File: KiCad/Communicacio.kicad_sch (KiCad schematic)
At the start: 11 parts, among them J2 USB_B_Micro, J3 Conn_PIC_ICSP_ICD, SW2 SW_SPDT, SW3 SW_SPDT, SW4 SW_SPDT, SW5 SW_SPDT, SW6 SW_SPDT, U5 FT232RL

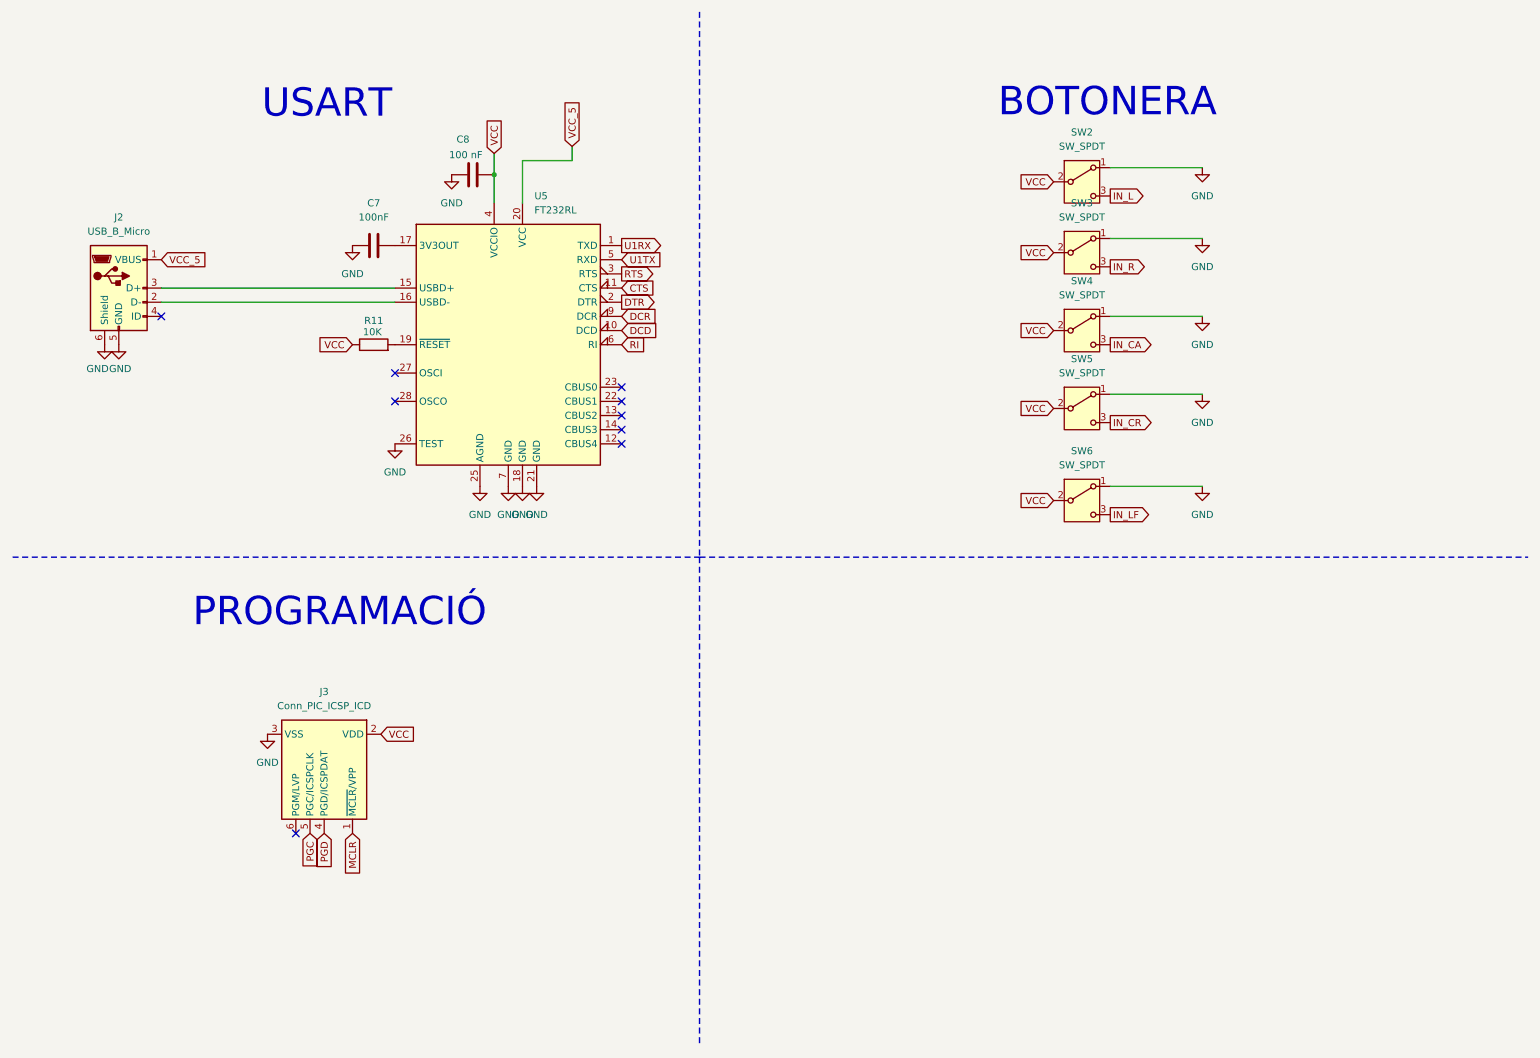
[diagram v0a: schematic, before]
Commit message: Debugging
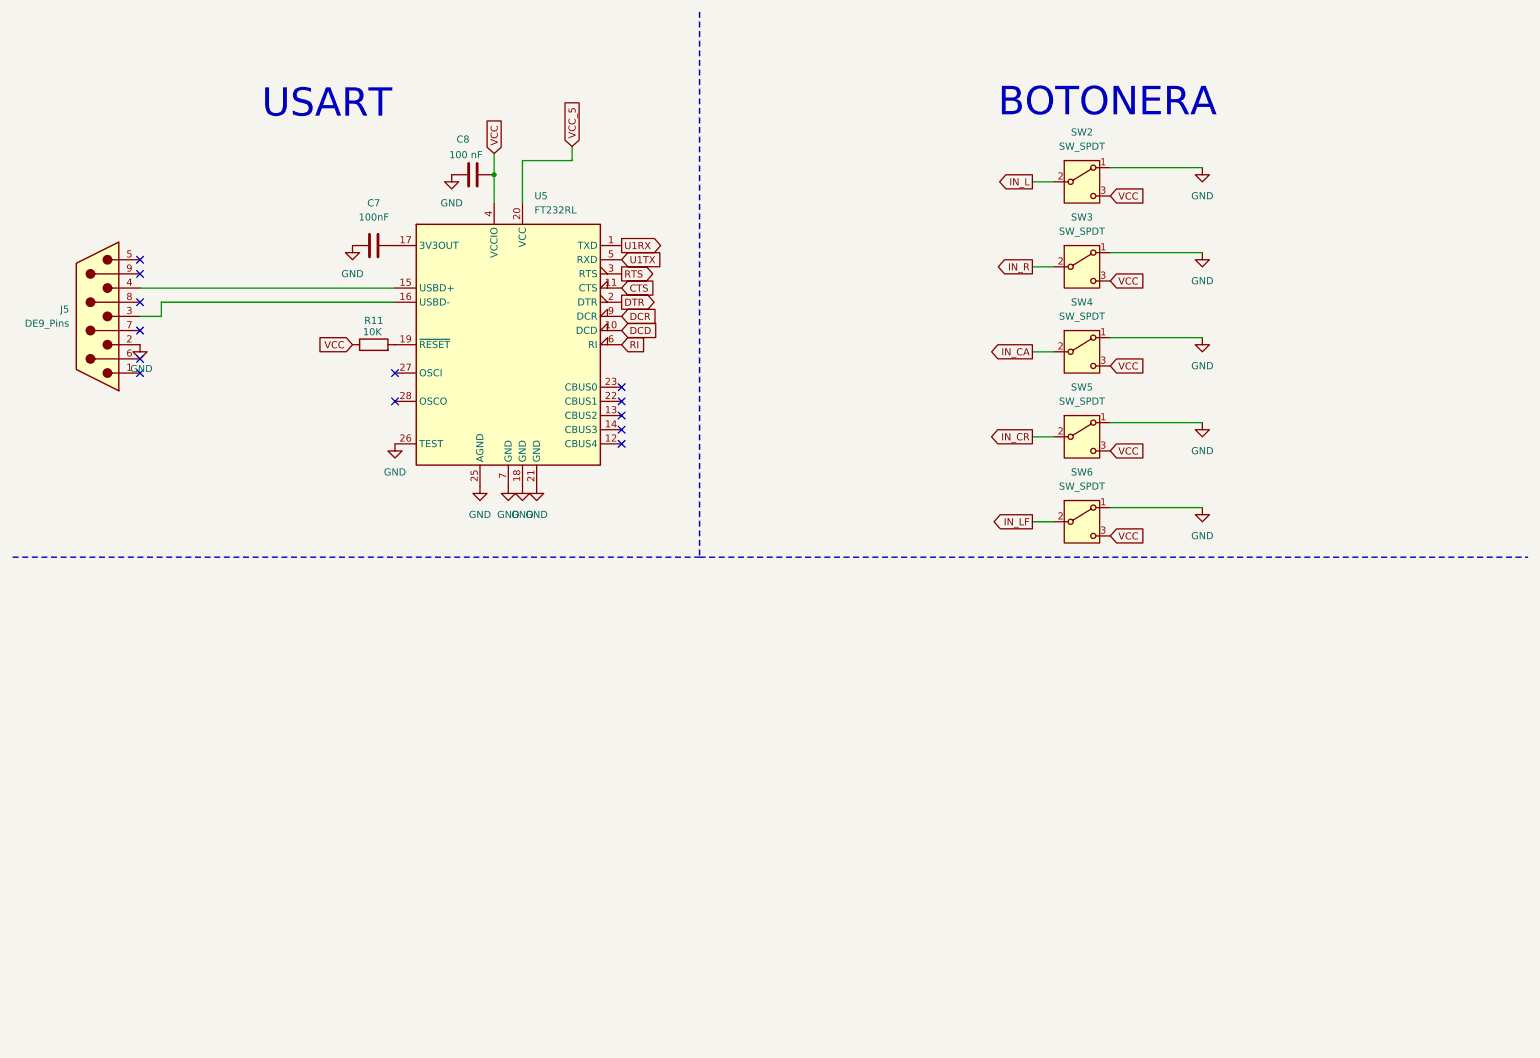
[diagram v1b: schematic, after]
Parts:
- removed J2: USB_B_Micro, symbol Connector:USB_B_Micro
- removed J3: Conn_PIC_ICSP_ICD, symbol Connector:Conn_PIC_ICSP_ICD
- added J5: DE9_Pins, symbol Connector:DE9_Pins
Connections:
- net GND: now also J5.2
- net IN_CA: now also SW4.2 (B); no longer SW4.3 (C)
- net IN_CR: now also SW5.2 (B); no longer SW5.3 (C)
- net IN_L: now also SW2.2 (B); no longer SW2.3 (C)
- net IN_LF: now also SW6.2 (B); no longer SW6.3 (C)
- net IN_R: now also SW3.2 (B); no longer SW3.3 (C)
- net VCC: now also SW2.3 (C), SW3.3 (C), SW4.3 (C), SW5.3 (C), SW6.3 (C); no longer SW2.2 (B), SW3.2 (B), SW4.2 (B), SW5.2 (B), SW6.2 (B)
- net at U5.16 (USBD-): now also J5.3
- net at U5.15 (USBD+): now also J5.4
- no-connect marks 9 -> 13
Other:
- note removed: "PROGRAMACIÓ"
